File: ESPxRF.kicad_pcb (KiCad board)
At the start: 4 copper layers, 22 parts, among them J1 Conn_Coaxial, J2 USB_C_Receptacle_USB2.0, U1 ESP32-S3, U2 NRF24L01, U3 NCP115ASN330T2G, U4 USBLC6-2SC6

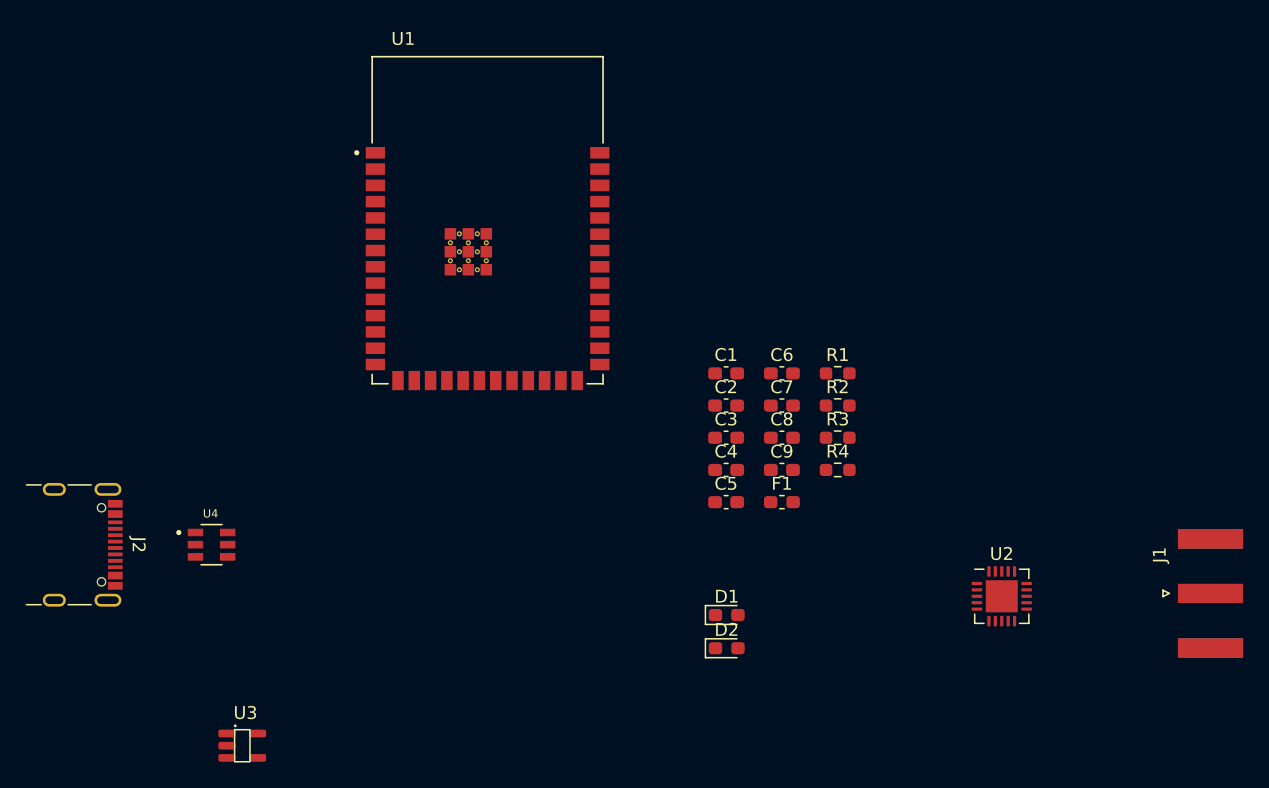
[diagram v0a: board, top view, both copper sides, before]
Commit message: nearly finished V1
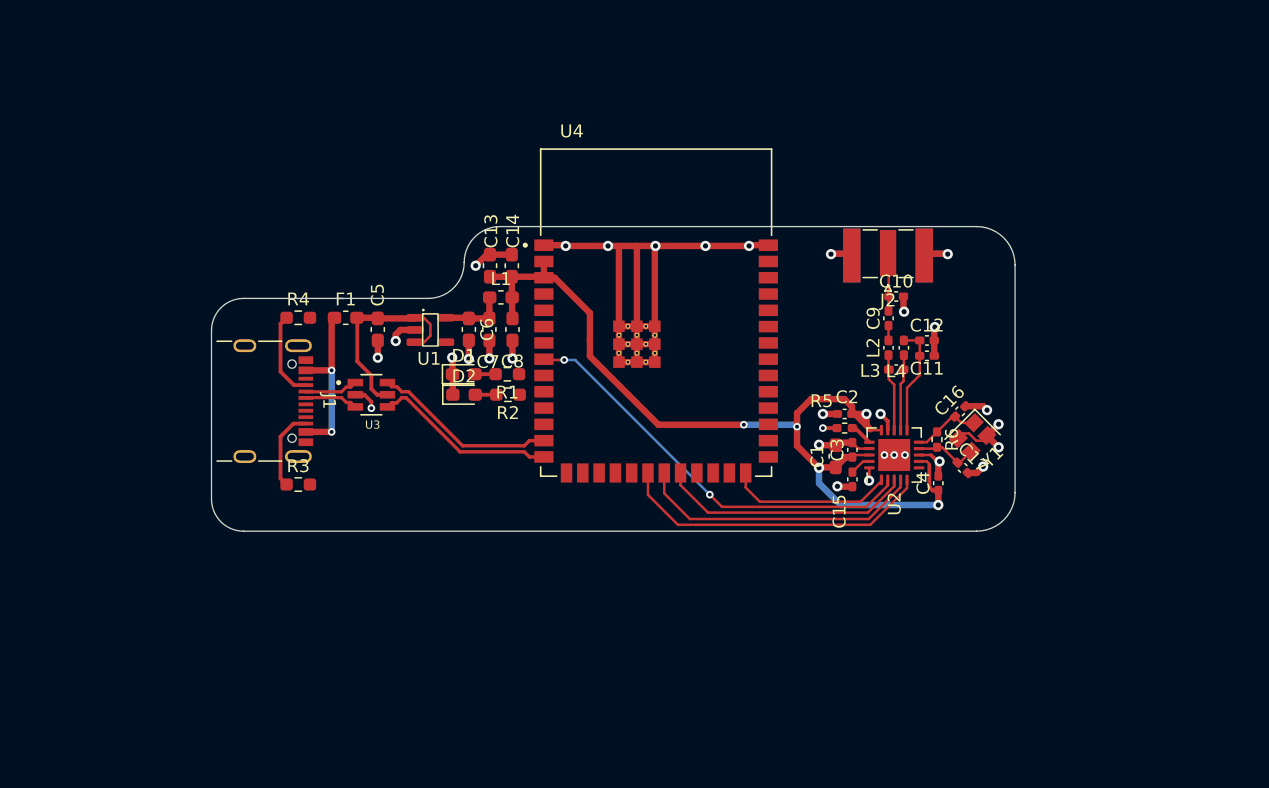
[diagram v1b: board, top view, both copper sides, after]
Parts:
- added C10: 1p, Capacitor_SMD:C_0402_1005Metric_Pad0.74x0.62mm_HandSolder, F.Cu at (139.7, 64.7)
- added C11: 2n2, Capacitor_SMD:C_0402_1005Metric_Pad0.74x0.62mm_HandSolder, F.Cu at (142.1, 69.3)
- added C12: 4p7, Capacitor_SMD:C_0402_1005Metric_Pad0.74x0.62mm_HandSolder, F.Cu at (142.1, 68.1)
- added C13: 10u, Capacitor_SMD:C_0603_1608Metric_Pad1.08x0.95mm_HandSolder, F.Cu at (108.0, 62.3)
- added C14: 100n, Capacitor_SMD:C_0603_1608Metric_Pad1.08x0.95mm_HandSolder, F.Cu at (109.7, 62.3)
- added C15: 33n, Capacitor_SMD:C_0402_1005Metric_Pad0.74x0.62mm_HandSolder, F.Cu at (136.3, 79.0)
- added C16: 22p, Capacitor_SMD:C_0402_1005Metric_Pad0.74x0.62mm_HandSolder, F.Cu at (144.7, 73.7)
- added C17: 22p, Capacitor_SMD:C_0402_1005Metric_Pad0.74x0.62mm_HandSolder, F.Cu at (144.9, 78.1)
- added L1: 100R @ 100MHz, Inductor_SMD:L_0603_1608Metric_Pad1.05x0.95mm_HandSolder, F.Cu at (108.9, 64.8)
- added L2: 3n9, Inductor_SMD:L_0402_1005Metric_Pad0.77x0.64mm_HandSolder, F.Cu at (139.1, 68.7)
- added L3: 8n2, Inductor_SMD:L_0402_1005Metric_Pad0.77x0.64mm_HandSolder, F.Cu at (139.7, 70.4)
- added L4: 2n7, Inductor_SMD:L_0402_1005Metric_Pad0.77x0.64mm_HandSolder, F.Cu at (140.3, 68.7)
- added R5: 22k, Resistor_SMD:R_0402_1005Metric_Pad0.72x0.64mm_HandSolder, F.Cu at (135.7, 75.0)
- added R6: 1M, Resistor_SMD:R_0402_1005Metric_Pad0.72x0.64mm_HandSolder, F.Cu at (142.9, 75.9)
- added Y1: Crystal_GND24_Small, Crystal:Crystal_SMD_2520-4Pin_2.5x2.0mm, F.Cu at (145.6, 75.7)
- C2, C3, C4: value 10u -> 100n; footprint Capacitor_SMD:C_0603_1608Metric_Pad1.08x0.95mm_HandSolder -> Capacitor_SMD:C_0402_1005Metric_Pad0.74x0.62mm_HandSolder
- C5, C6: value 100n -> 10u
- C9: value 100n -> 1p5; footprint Capacitor_SMD:C_0603_1608Metric_Pad1.08x0.95mm_HandSolder -> Capacitor_SMD:C_0402_1005Metric_Pad0.74x0.62mm_HandSolder
- F1: value 100mA -> 500mA
- J1: value Conn_Coaxial -> USB_C_Receptacle_USB2.0; footprint Connector_Coaxial:SMA_Amphenol_132289_EdgeMount -> Connector_USB:USB_C_Receptacle_GCT_USB4105-xx-A_16P_TopMnt_Horizontal
- J2: value USB_C_Receptacle_USB2.0 -> ANT; footprint Connector_USB:USB_C_Receptacle_GCT_USB4105-xx-A_16P_TopMnt_Horizontal -> Connector_Coaxial:SMA_Samtec_SMA-J-P-X-ST-EM1_EdgeMount
- R1, R2: value 5k1 -> 1k3
- R3, R4: value 1k3 -> 5k1
- U1: value ESP32-S3 -> NCP115ASN330T2G; footprint ESP32:XCVR_ESP32S3WROOM1N8R8 -> NCP115ASN330T2G:NCP115ASN330T2G
- U3: value NCP115ASN330T2G -> USBLC6-2SC6; footprint NCP115ASN330T2G:NCP115ASN330T2G -> SnapEda:SOT95P280X145-6N
- U4: value USBLC6-2SC6 -> ESP32-S3; footprint SnapEda:SOT95P280X145-6N -> ESP32:XCVR_ESP32S3WROOM1N8R8
- moved J1 75.7 mm to (90.0, 72.9), turned to -90 degrees
- moved J2 67.8 mm to (139.1, 61.5), turned to 180 degrees
- moved R4 43.7 mm to (93.1, 66.4)
- moved R3 42.2 mm to (93.1, 79.4)
- moved U4 39.1 mm to (121.0, 66.0)
- moved F1 36.9 mm to (96.8, 66.4)
- moved C5 30.3 mm to (99.3, 67.3), turned to -90 degrees
- moved U3 29.2 mm to (98.8, 72.4)
- moved D2 28.5 mm to (106.0, 72.4)
- moved D1 27.8 mm to (106.0, 70.8)
- moved R1 25.8 mm to (109.4, 70.8), turned to 180 degrees
- moved R2 25.7 mm to (109.4, 72.4), turned to 180 degrees
- moved C6 24.6 mm to (106.4, 67.3), turned to -90 degrees
- moved C7 23.6 mm to (108.0, 67.3), turned to -90 degrees
- moved C8 22.6 mm to (109.8, 67.3), turned to -90 degrees
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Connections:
- C1 pad 1: +5V -> +3V3
- C5 pad 1: +3V3 -> +5V
- C6 pad 1: +3V3 -> Net-(U1-out)
- C7 pad 1: +3V3 -> Net-(U1-out)
- C9 pad 1: GND -> Net-(C9-Pad1)
- C9 pad 2: Net-(J2-SHIELD) -> Net-(J2-In)
- R1 pad 1: Net-(J2-CC2) -> Net-(U4-IO16)
- R1 pad 2: GND -> Net-(D1-A)
- R2 pad 1: Net-(J2-CC1) -> Net-(U4-IO17)
- R2 pad 2: GND -> Net-(D2-A)
- R3 pad 1: unconnected-(R3-Pad1) -> Net-(J1-CC2)
- R3 pad 2: Net-(D1-A) -> GND
- R4 pad 1: unconnected-(R4-Pad1) -> Net-(J1-CC1)
- R4 pad 2: Net-(D2-A) -> GND
- U1 pad 1: GND -> +5V
- U1 pad 2: +3V3 -> GND
- U1 pad 3: unconnected-(U1-EN-Pad3) -> +5V
- U1 pad 4: unconnected-(U1-IO4-Pad4) -> (no net)
- U1 pad 5: unconnected-(U1-IO5-Pad5) -> Net-(U1-out)
- U2 pad 1: unconnected-(U2-CE-Pad1) -> CE
- U2 pad 10: unconnected-(U2-XC1-Pad10) -> XC1
- U2 pad 11: unconnected-(U2-VDD_PA-Pad11) -> VDD_PA
- U2 pad 12: unconnected-(U2-ANT1-Pad12) -> ANT1
- U2 pad 13: unconnected-(U2-ANT2-Pad13) -> ANT2
- U2 pad 16: unconnected-(U2-IREF-Pad16) -> Net-(U2-IREF)
- U2 pad 19: unconnected-(U2-DVDD-Pad19) -> Net-(U2-DVDD)
- U2 pad 2: unconnected-(U2-CSN-Pad2) -> CSN
- U2 pad 3: unconnected-(U2-SCK-Pad3) -> SCK
- U2 pad 4: unconnected-(U2-MOSI-Pad4) -> MOSI
- U2 pad 5: unconnected-(U2-MISO-Pad5) -> MISO
- U2 pad 6: unconnected-(U2-IRQ-Pad6) -> IRQ
- U2 pad 9: unconnected-(U2-XC2-Pad9) -> XC2
- U3 pad 1: +5V -> USBCON_D-
- U3 pad 3: +5V -> USBCON_D+
- U3 pad 4: (no net) -> USB_D+
- U3 pad 5: +3V3 -> +5V
- U4 pad 1: unconnected-(U4-Pad1) -> GND
- U4 pad 2: GND -> +3V3
- U4 pad 3: unconnected-(U4-Pad3) -> +3V3
- U4 pad 5: +5V -> unconnected-(U4-IO5-Pad5)
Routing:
- net GND: track 0.00 -> 102.8 mm, vias 0 -> 31
- net +3V3: track 0.00 -> 71.5 mm, vias 0 -> 5
- net CSN: track 0.00 -> 32.7 mm, vias 0 -> 2
- net MISO: track 0.00 -> 24.7 mm
- net MOSI: track 0.00 -> 22.4 mm
- net SCK: track 0.00 -> 19.8 mm
- net +5V: track 0.00 -> 15.7 mm
- net USB_D-: track 0.00 -> 14.4 mm
- net USB_D+: track 0.00 -> 14.4 mm
- net Net-(F1-Pad1): track 0.00 -> 13.0 mm, vias 0 -> 2
- net CE: track 0.00 -> 12.9 mm
- net VDD_PA: track 0.00 -> 8.64 mm
- net Net-(J1-CC1): track 0.00 -> 6.81 mm
- net Net-(J1-CC2): track 0.00 -> 6.33 mm
- net ANT2: track 0.00 -> 6.03 mm
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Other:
- board outline added: 62.6 x 23.8 mm
- board text added: "RX"
- board text added: "TX"
